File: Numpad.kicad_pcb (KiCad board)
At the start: 2 copper layers, 76.2 x 97.6 mm, 51 parts, among them J1 USB_B_Mini, SW0 0, SW1 1, SW2 2, SW3 3, SW4 4, SW5 5, SW6 6, SW7 7, SW8 8, SW9 9, U1 ATmega32U4-AU, Y1 16MHz

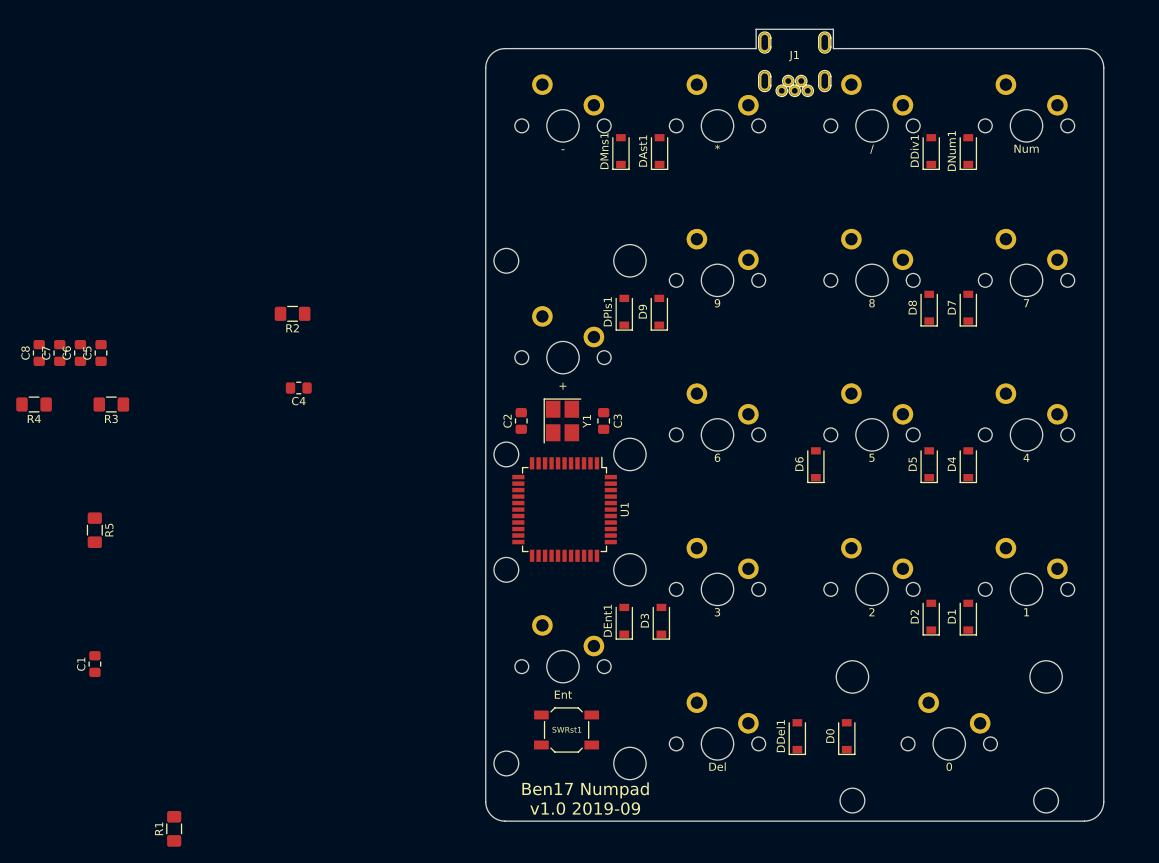
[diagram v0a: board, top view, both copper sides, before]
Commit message: plate files added, moved around some more components
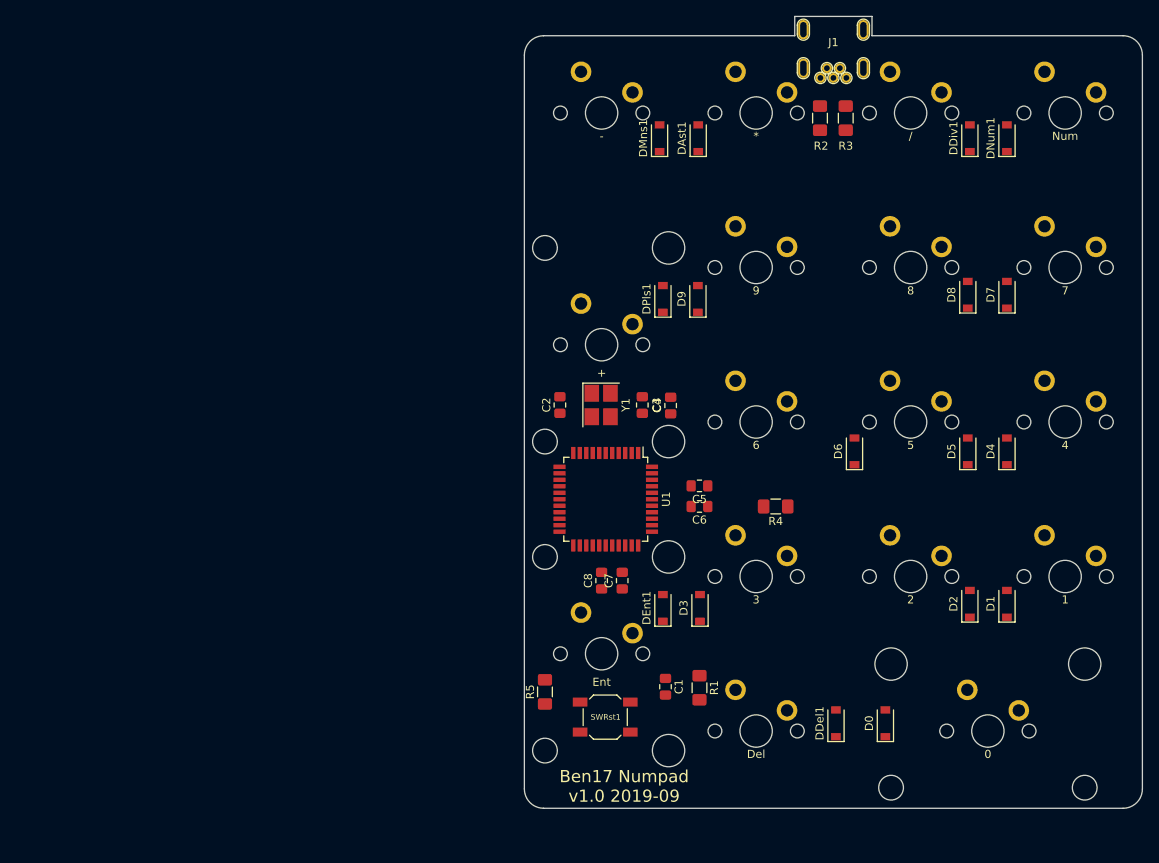
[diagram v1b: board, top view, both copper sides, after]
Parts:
- moved R3 97.2 mm to (197.7, 49.5), turned to 90 degrees
- moved R4 92.3 mm to (189.1, 97.4)
- moved C6 78.6 mm to (179.7, 97.4), turned to 180 degrees
- moved C5 75.6 mm to (179.7, 94.9), turned to 180 degrees
- moved C7 74.8 mm to (170.2, 106.6)
- moved C8 74.8 mm to (167.6, 106.6)
- moved C1 70.4 mm to (175.5, 119.6), turned to 270 degrees
- moved R2 69.4 mm to (194.6, 49.5), turned to 90 degrees
- moved R1 67.1 mm to (179.7, 119.8), turned to 270 degrees
- moved R5 59.0 mm to (160.7, 120.3), turned to 90 degrees
- moved C4 45.9 mm to (176.1, 85.0), turned to 90 degrees
- moved U1 5.24 mm to (168.1, 96.5)
- moved Y1 5.15 mm to (167.6, 84.9)
- moved C2 5.15 mm to (162.5, 84.9)
- moved C3 5.15 mm to (172.7, 84.9)
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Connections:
- U1 pad 10: Row3 -> Net-(U1-Pad10)
- U1 pad 11: Row4 -> Net-(U1-Pad11)
- U1 pad 18: Col1 -> Net-(U1-Pad18)
- U1 pad 19: Col2 -> Net-(U1-Pad19)
- U1 pad 20: Col3 -> Net-(U1-Pad20)
- U1 pad 21: Col4 -> Net-(U1-Pad21)
- U1 pad 25: Net-(U1-Pad25) -> Col4
- U1 pad 26: Net-(U1-Pad26) -> Col3
- U1 pad 28: Row5 -> Col2
- U1 pad 29: Net-(U1-Pad29) -> Col1
- U1 pad 37: Net-(U1-Pad37) -> Row5
- U1 pad 38: Net-(U1-Pad38) -> Row4
- U1 pad 39: Net-(U1-Pad39) -> Row3
- U1 pad 40: Net-(U1-Pad40) -> Row2
- U1 pad 41: Net-(U1-Pad41) -> Row1
- U1 pad 8: Row1 -> Net-(U1-Pad8)
- U1 pad 9: Row2 -> Net-(U1-Pad9)
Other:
- net class Power added: clearance 0.2, trace_width 0.381, via_dia 0.8, via_drill 0.4
